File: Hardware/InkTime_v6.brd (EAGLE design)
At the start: 46 x 35 mm, 105 parts, among them IC1 DRV2605YZFR, IC2 BQ25180YBGR, IC3 BMA421, IC9 RT6160AWSC, J1 KH-TYPE-C-16P, J2 503480-2400, J3 TC2030-IDC, Q3 SI1308EDL-T1-GE3, U1 MAX17048G+T10, U2 NRF52840_QF, X1 32MHz, X2 32.768kHz

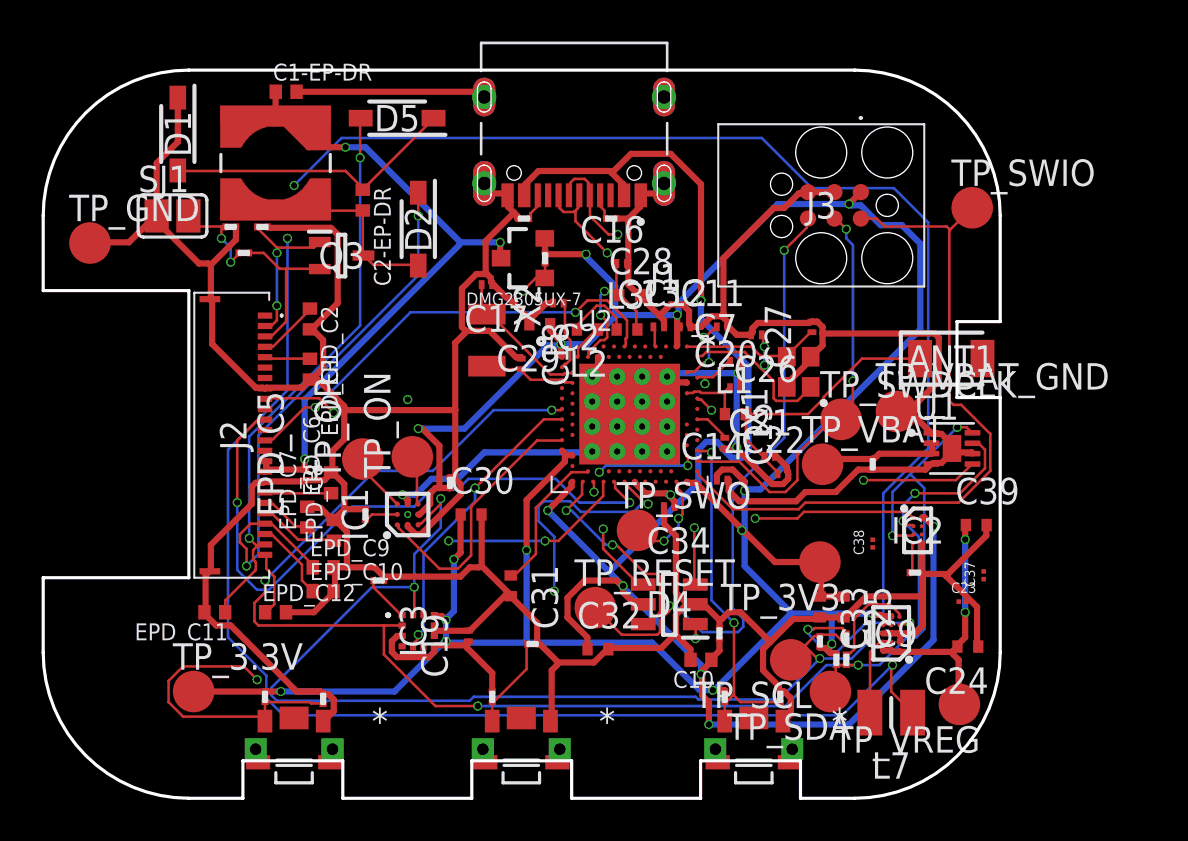
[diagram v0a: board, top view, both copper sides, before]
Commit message: PCB finalizat
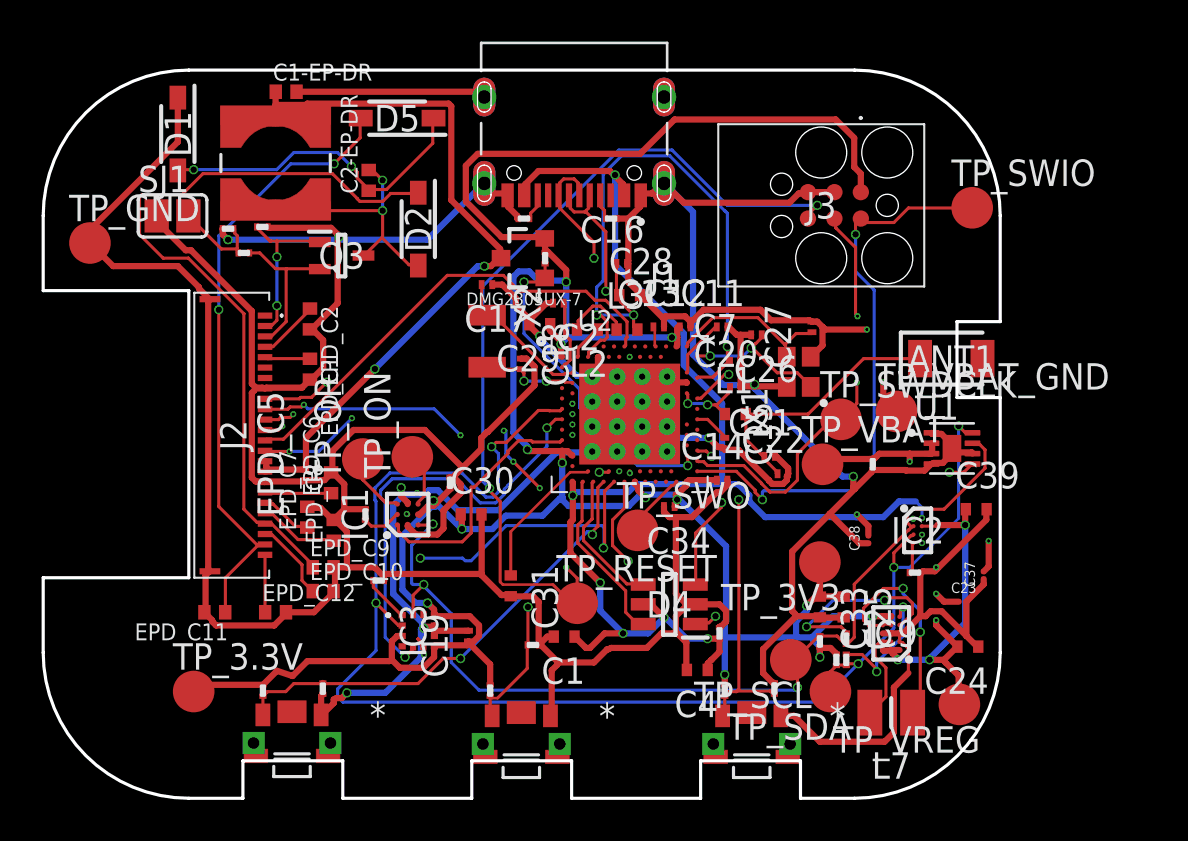
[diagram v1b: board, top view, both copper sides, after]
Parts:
- C1: value 1uF -> 4.7μF; device Library_proiect:GRM011R60J152KE01L_1_0201 -> InkTime_v5:NORDIC_NRF_3_RESC0402_L
- C10: value 4.7uF -> 1uF; device Library_proiect:PERFECT_0402_0402 -> Library_proiect:GRM011R60J152KE01L_1_0201
- C29: device InkTime_v5:NORDIC_NRF_3_RESC0402_L -> Library_proiect:NORDIC_NRF_3_RESC0402_L
- C32: value 4.7μF -> 1uF; device InkTime_v5:NORDIC_NRF_3_RESC0402_L -> Library_proiect:GRM011R60J152KE01L_1_0201
- C4: value 1uF -> 4.7uF; device Library_proiect:GRM011R60J152KE01L_1_0201 -> InkTime_v5:NORDIC_NRF_3_RESC0402_L
- X2: device InkTime_v5:NORDIC_NRF_1_XTAL_3215_N -> Library_proiect:NORDIC_NRF_1_XTAL_3215_N
- moved C5 22.0 mm to (64.5, 43.7), turned to 180 degrees
- moved C1 12.0 mm to (76.1, 46.2), turned to 180 degrees
- moved C32 8.69 mm to (86.2, 43.7)
- moved C10 8.11 mm to (74.6, 45.8), turned to 270 degrees
- moved C4 8.02 mm to (82.5, 44.6), turned to 180 degrees
- moved C2-EP-DR 0.99 mm to (66.7, 68.1), turned to 90 degrees
- moved TP_RESET 0.89 mm to (76.7, 47.8)
- moved C39 0.76 mm to (95.9, 52.3)
- moved R8 0.32 mm to (72.5, 43.6)
- moved R5 0.32 mm to (61.6, 43.6)
- moved SW_UP 0.32 mm to (63.0, 41.5)
- moved R7 0.30 mm to (83.8, 43.6)
- moved C38 0.29 mm to (90.7, 50.9)
- moved SW_DN 0.27 mm to (85.1, 41.4)
- moved SW_ENT 0.25 mm to (74.0, 41.4)
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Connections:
- net GND: now also C1.2, C10.1, C32.1, C4.2; no longer C1.1, C10.2, C32.2, C4.1
- net P0.13: now also C5.2; no longer C1.2
- net P0.14: now also C10.2; no longer C4.2
- net P1.02: now also C32.2; no longer C5.2
- net VBUS: now also C1.1, C4.1; no longer C10.1, C32.1
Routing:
- net LX2: track 67.5 -> 10.9 mm
- net GND: track 284.0 -> 339.8 mm, vias 3 -> 13
- net N$17: track 64.7 -> 9.17 mm, vias 3 -> 2
- net PMIC_INT: track 48.7 -> 18.4 mm
- net D-: track 30.8 -> 8.43 mm, vias 2 -> 0
- net D+: track 27.7 -> 6.77 mm, vias 2 -> 0
- net EPD_RST: track 0.00 -> 20.0 mm, vias 0 -> 6
- net MOSI: track 0.00 -> 19.4 mm, vias 0 -> 3
- net 3V3: track 154.4 -> 135.8 mm, vias 16 -> 14
- net VBUS: track 79.8 -> 63.1 mm, vias 6 -> 8
- net IMU_INT2: track 0.00 -> 15.8 mm, vias 0 -> 2
- net EPD_CS: track 0.00 -> 15.4 mm, vias 0 -> 2
- net P0.13: track 36.9 -> 23.0 mm, vias 3 -> 2
- net SCL: track 68.3 -> 56.0 mm, vias 5 -> 4
- net P0.14: track 4.45 -> 14.7 mm, vias 0 -> 2
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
